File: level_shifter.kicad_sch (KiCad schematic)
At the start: 2 parts, among them U10 SN74AHC1G125DBVR

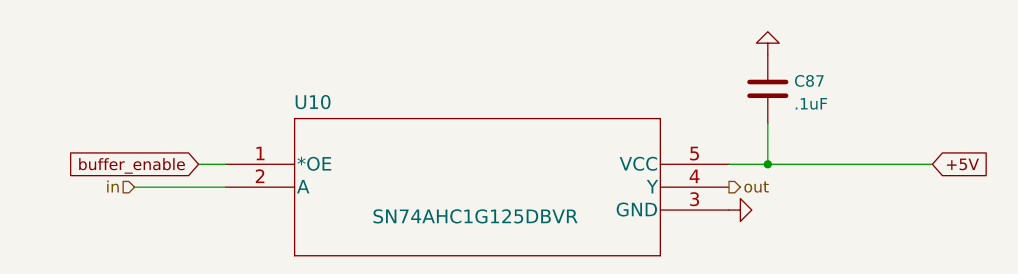
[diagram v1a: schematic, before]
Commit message: All DRC errors cleared after conversion to Kicad V7
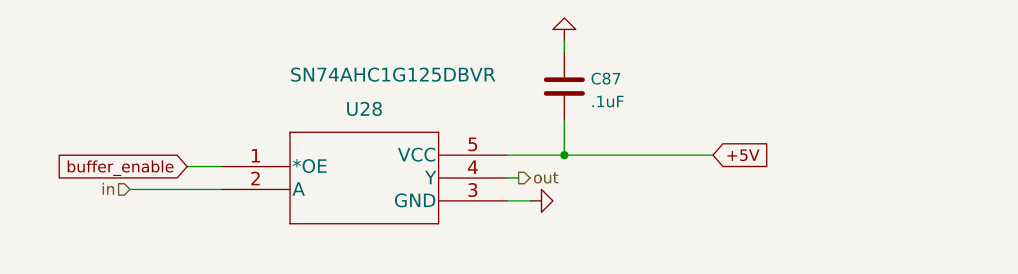
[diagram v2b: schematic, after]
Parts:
- removed U10: SN74AHC1G125DBVR, Project_Footprints_Library:SN74AHC1G125DBVR, symbol 1LibBBCTRL:SN74AHC1G125DBVR
- added U28: SN74AHC1G125DBVR, Project_Footprints_Library:SN74AHC1G125DBVR, symbol 1LibBBCTRL:SN74AHC1G125DBVR
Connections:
- net +5V: now also U28.5 (VCC)
- net GND: now also U28.3 (GND)
- net buffer_enable: now also U28.1 (*OE)
- net in: now also U28.2 (A)
- net out: now also U28.4 (Y)
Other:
- moved on the sheet: C87
